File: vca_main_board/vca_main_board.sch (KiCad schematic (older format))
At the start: 0 parts

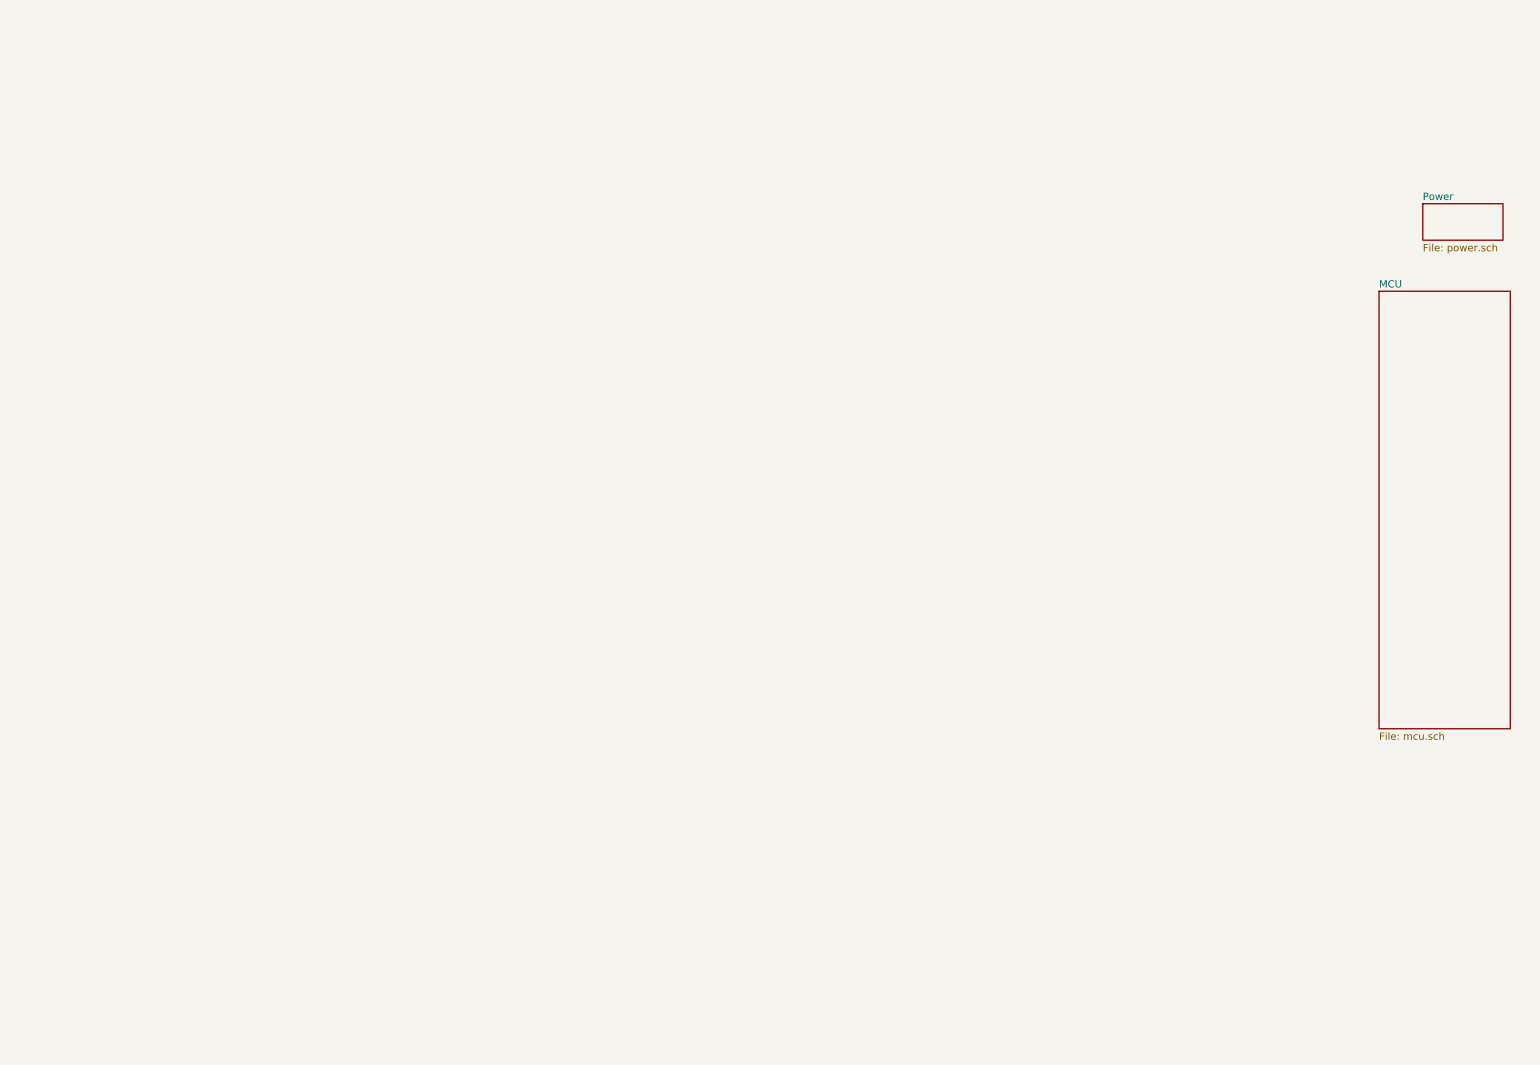
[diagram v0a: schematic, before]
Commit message: done
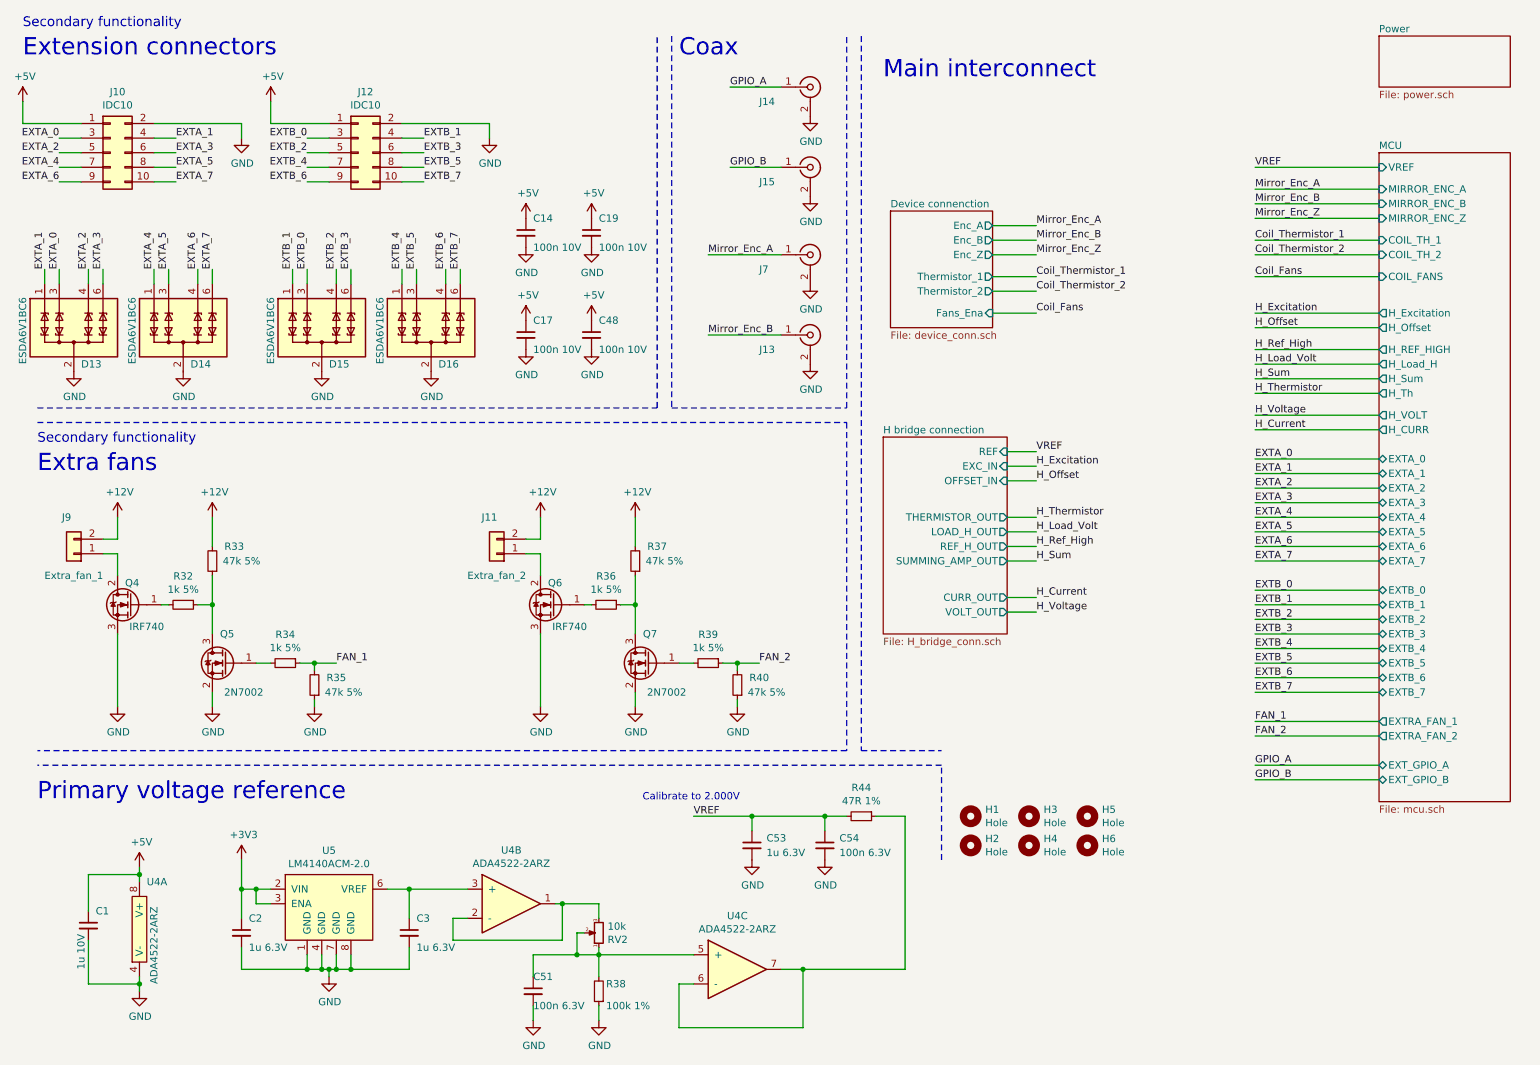
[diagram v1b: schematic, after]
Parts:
- added C1: 1u 10V, Capacitor_SMD:C_0603_1608Metric_Pad1.08x0.95mm_HandSolder, symbol Device:C_Small
- added C14, C17, C19, C48: 100n 10V, Capacitor_SMD:C_0603_1608Metric_Pad1.08x0.95mm_HandSolder, symbol Device:C_Small
- added C2, C3, C53: 1u 6.3V, Capacitor_SMD:C_0603_1608Metric_Pad1.08x0.95mm_HandSolder, symbol Device:C_Small
- added C51, C54: 100n 6.3V, Capacitor_SMD:C_0603_1608Metric_Pad1.08x0.95mm_HandSolder, symbol Device:C_Small
- added D13, D14, D15, D16: ESDA6V1BC6, Package_TO_SOT_SMD:SOT-23-6, symbol Power_Protection:ESDA6V1BC6
- added H1, H2, H3, H4, H5, H6: Hole, MountingHole:MountingHole_3.2mm_M3_Pad_Via, symbol Mechanical:MountingHole
- added J10, J12: IDC10, Connector_IDC:IDC-Header_2x05_P2.54mm_Vertical, symbol Connector_Generic:Conn_02x05_Odd_Even
- added J11: Extra_fan_2, Connector_PinHeader_2.54mm:PinHeader_1x02_P2.54mm_Vertical, symbol Connector_Generic:Conn_01x02
- added J13, J14, J15, J7: Conn_Coaxial, 1-1634613-0:1-1634613-0, symbol Connector:Conn_Coaxial
- added J9: Extra_fan_1, Connector_PinHeader_2.54mm:PinHeader_1x02_P2.54mm_Vertical, symbol Connector_Generic:Conn_01x02
- added Q4, Q6: IRF740, Package_TO_SOT_THT:TO-220-3_Horizontal_TabDown, symbol Transistor_FET:IRF740
- added Q5, Q7: 2N7002, Package_TO_SOT_SMD:SOT-23, symbol Transistor_FET:2N7002
- added R32, R34, R36, R39: 1k 5%, Resistor_SMD:R_0603_1608Metric_Pad0.98x0.95mm_HandSolder, symbol Device:R_Small
- added R33, R35, R37, R40: 47k 5%, Resistor_SMD:R_0603_1608Metric_Pad0.98x0.95mm_HandSolder, symbol Device:R_Small
- added R38: 100k 1%, Resistor_SMD:R_0603_1608Metric_Pad0.98x0.95mm_HandSolder, symbol Device:R_Small
- added R44: 47R 1%, Resistor_SMD:R_0603_1608Metric_Pad0.98x0.95mm_HandSolder, symbol Device:R_Small
- added RV2: 10k, Bourns_3214W:Bourns_3214W, symbol Device:R_POT_Small
- added U4: ADA4522-2ARZ, Package_SO:SOIC-8_3.9x4.9mm_P1.27mm, symbol ADA4522-2:ADA4522-2ARZ
- added U5: LM4140ACM-2.0, Package_SO:SOIC-8_3.9x4.9mm_P1.27mm, symbol LM4140ACM-2.0:LM4140ACM-2.0
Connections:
- new net: C51.1, R38.2, RV2.1, RV2.2, U4.5 (+)
- new net: RV2.3, U4.1, U4.2 (-)
- new net: R44.1, U4.6 (-), U4.7
- new net: Q4.1 (G), R32.2
- new net: J9.1 (Pin_1), Q4.2 (D)
- new net: Q5.1 (G), R34.2
- new net: Q5.3 (D), R32.1, R33.1
- new net: Q6.1 (G), R36.2
- new net: J11.1 (Pin_1), Q6.2 (D)
- new net: Q7.1 (G), R39.2
- new net: Q7.3 (D), R36.1, R37.1
- new net: C3.1, U4.3 (+), U5.6 (VREF)
- new net +12V: J11.2 (Pin_2), J9.2 (Pin_2), R33.2, R37.2
- new net +3V3: C2.1, U5.2 (VIN), U5.3 (ENA)
- new net +5V: C1.1, C14.1, C17.1, C19.1, C48.1, J10.1 (Pin_1), J12.1 (Pin_1), U4.8 (V+)
- new net EXTA_0: D13.3 (TVS2), J10.3 (Pin_3)
- new net EXTA_1: D13.1 (TVS1), J10.4 (Pin_4)
- new net EXTA_2: D13.4 (TVS3), J10.5 (Pin_5)
- new net EXTA_3: D13.6 (TVS4), J10.6 (Pin_6)
- new net EXTA_4: D14.1 (TVS1), J10.7 (Pin_7)
- new net EXTA_5: D14.3 (TVS2), J10.8 (Pin_8)
- new net EXTA_6: D14.4 (TVS3), J10.9 (Pin_9)
- new net EXTA_7: D14.6 (TVS4), J10.10 (Pin_10)
- new net EXTB_0: D15.3 (TVS2), J12.3 (Pin_3)
- new net EXTB_1: D15.1 (TVS1), J12.4 (Pin_4)
- new net EXTB_2: D15.4 (TVS3), J12.5 (Pin_5)
- new net EXTB_3: D15.6 (TVS4), J12.6 (Pin_6)
- new net EXTB_4: D16.1 (TVS1), J12.7 (Pin_7)
- new net EXTB_5: D16.3 (TVS2), J12.8 (Pin_8)
- new net EXTB_6: D16.4 (TVS3), J12.9 (Pin_9)
- new net EXTB_7: D16.6 (TVS4), J12.10 (Pin_10)
- new net FAN_1: R34.1, R35.2
- new net FAN_2: R39.1, R40.2
- new net GND: C1.2, C14.2, C17.2, C19.2, C2.2, C3.2, C48.2, C51.2, C53.2, C54.2, D13.2 (COM), D13.5 (COM), D14.2 (COM), D14.5 (COM), D15.2 (COM), D15.5 (COM), D16.2 (COM), D16.5 (COM), J10.2 (Pin_2), J12.2 (Pin_2), J13.2 (Ext), J14.2 (Ext), J15.2 (Ext), J7.2 (Ext), Q4.3 (S), Q5.2 (S), Q6.3 (S), Q7.2 (S), R35.1, R38.1, R40.1, U4.4 (V-), U5.1 (GND), U5.4 (GND), U5.7 (GND), U5.8 (GND)
- new net GPIO_A: J14.1 (In)
- new net GPIO_B: J15.1 (In)
- new net Mirror_Enc_A: J7.1 (In)
- new net Mirror_Enc_B: J13.1 (In)
- new net VREF: C53.1, C54.1, R44.2
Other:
- note added: "Calibrate to 2.000V"
- note added: "Coax"
- note added: "Extension connectors"
- note added: "Extra fans"
- note added: "Main interconnect"
- note added: "Primary voltage reference"
- note added: "Secondary functionality"
